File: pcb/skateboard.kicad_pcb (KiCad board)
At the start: 4 copper layers, 86.2 x 84.8 mm, 177 parts, among them J1 RC555, J10 PH_2.0, J11 adc_sensor2, J12 adc_sensor1, J13 Conn_01x01_Pin, J14 Conn_01x01_Pin, J15 Conn_01x01_Pin, J16 Conn_01x01_Pin, J2 pa1010d, J3 can_sensor, J4 USB_C_Receptacle_USB2.0_16P, J5 UART, J6 TB_MOTOR, J7 PH_2.0, J8 power, J9 TB_MOTOR, Q1 AO3401A, Q4 BTN8982TA, Q5 BTN8982TA, Q6 BTN8982TA, Q7 BTN8982TA, Q8 BTN8982TA, Q9 BTN8982TA, SW1 SW_SPST, SW2 BOOT, SW3 EN, U1 HX711, U10 INA240A2PW, U11 INA240A2PW, U2 SIT1042AQT/3, U3 ESP32-S3-WROOM-1, U4 LMR16030SDDAR, U5 LMR16030SDDAR, U6 LMR16030SDDAR, U7 INA240A2PW, U8 INA240A2PW, U9 HX711

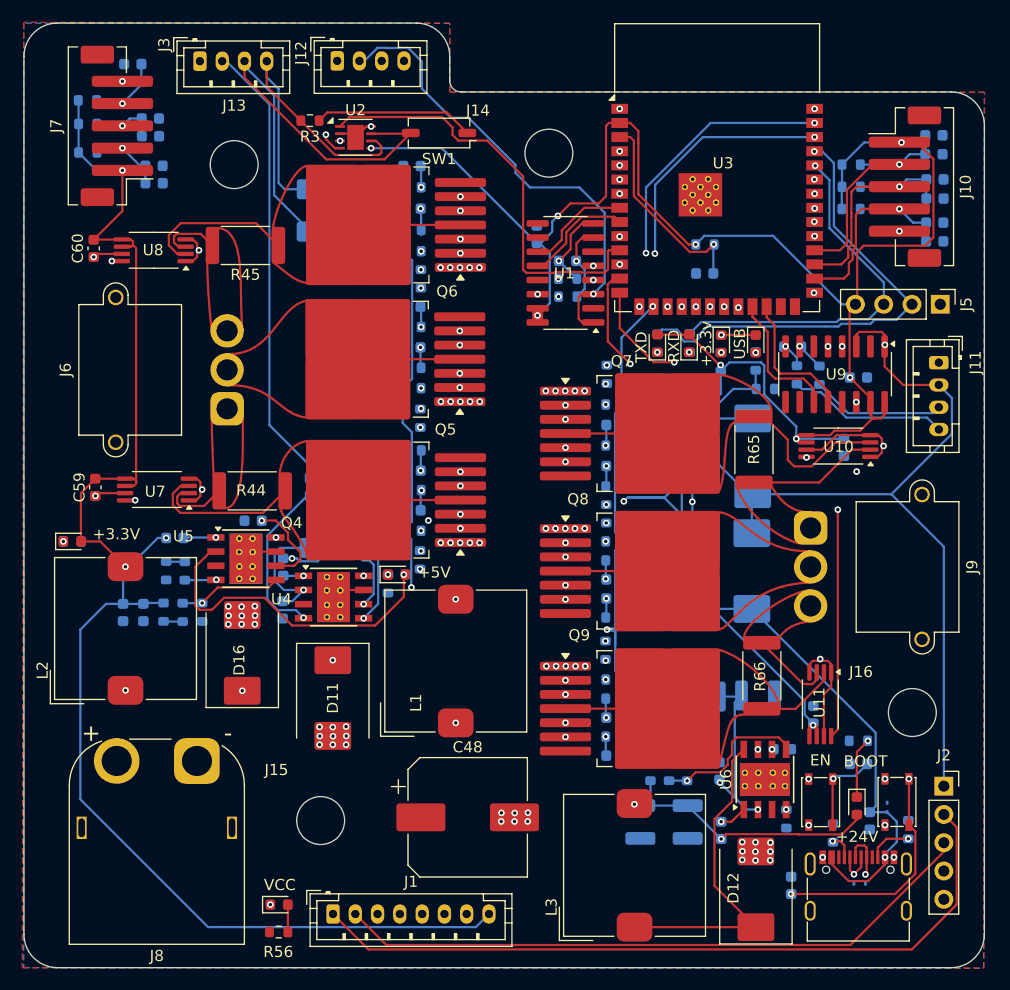
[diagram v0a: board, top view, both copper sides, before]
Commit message: update
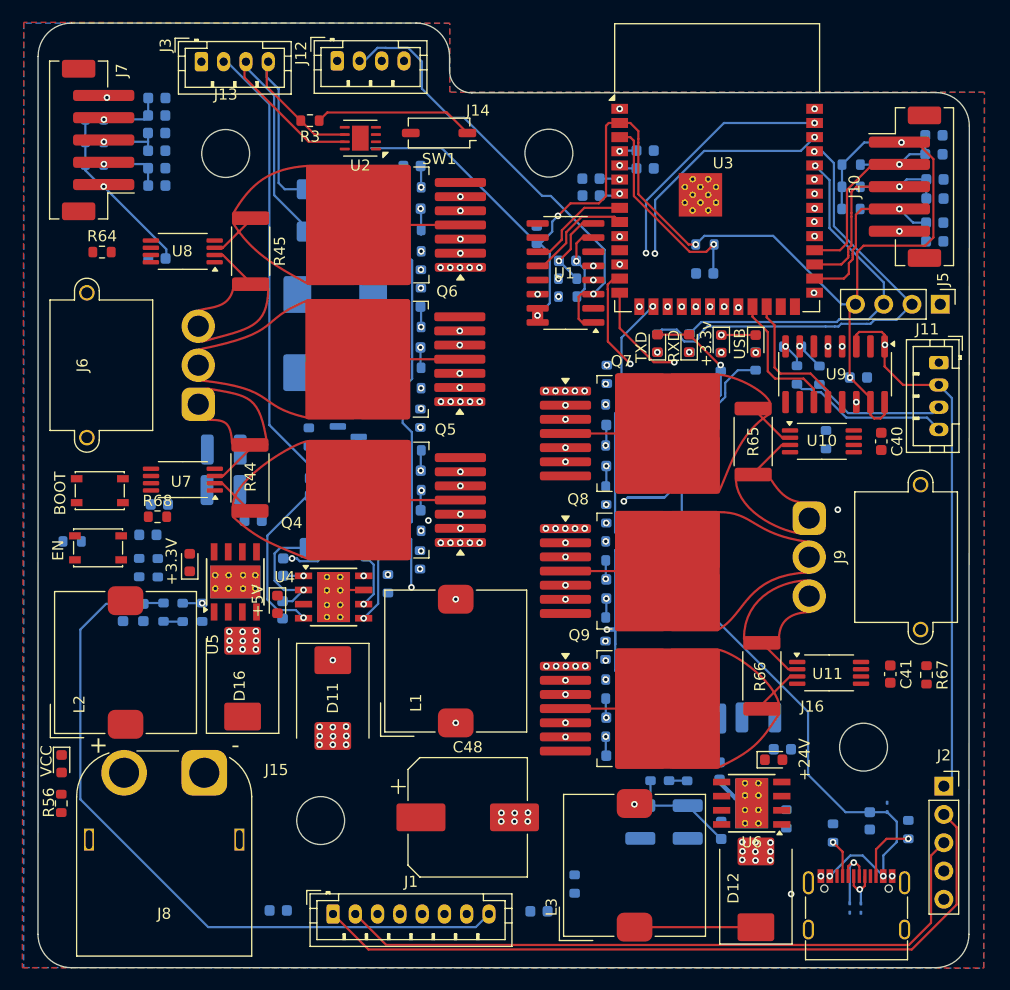
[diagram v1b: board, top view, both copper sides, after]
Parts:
- added C21: 100nf, Capacitor_SMD:C_0603_1608Metric, B.Cu at (137.9, 84.7)
- added C24: 100nf, Capacitor_SMD:C_0603_1608Metric, B.Cu at (142.8, 82.2)
- added C28: 100nf, Capacitor_SMD:C_0603_1608Metric, B.Cu at (137.9, 86.2)
- added C6: 100nf, Capacitor_SMD:C_0603_1608Metric, B.Cu at (142.8, 83.8)
- added R64: 200k, Resistor_SMD:R_0603_1608Metric, F.Cu at (94.0, 91.3)
- added R67: 200k, Resistor_SMD:R_0603_1608Metric, F.Cu at (168.1, 129.3)
- added R68: 200k, Resistor_SMD:R_0603_1608Metric, F.Cu at (99.0, 115.1)
- added R69: 200k, Resistor_SMD:R_0603_1608Metric, B.Cu at (159.0, 108.1)
- C12, C13, C19: value 100nF/16v -> 100nF
- C40, C41: moved to F.Cu
- C59, C60: moved to B.Cu
- C8: value 100nf/50v -> 100nf
- D4, D5: value MBR120VLSFT1G -> B560C
- moved SW2 76.8 mm to (93.8, 112.7), turned to 0 degrees
- moved SW3 68.8 mm to (93.7, 117.9), turned to 0 degrees
- moved C43 46.1 mm to (109.8, 150.4), turned to 0 degrees
- moved D4 41.4 mm to (115.0, 102.1), turned to 180 degrees
- moved C15 41.2 mm to (105.0, 109.0)
- moved C14 41.2 mm to (104.9, 112.7)
- moved R7 41.2 mm to (112.6, 107.9), turned to 90 degrees
- moved D5 40.2 mm to (115.0, 95.1), turned to 180 degrees
- moved C45 31.6 mm to (133.3, 150.5), turned to 0 degrees
- moved Q1 31.0 mm to (116.1, 107.9), turned to 0 degrees
- moved R19 28.5 mm to (136.5, 148.0), turned to -90 degrees
- moved 3.3V4 23.3 mm to (90.4, 137.2), turned to -90 degrees
- moved R56 22.7 mm to (90.4, 140.8), turned to 90 degrees
- moved D14 11.0 mm to (109.8, 122.9), turned to -90 degrees
- moved D17 10.7 mm to (101.9, 119.2), turned to 90 degrees
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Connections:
- Q4 pad 4: Net-(U7--) -> Net-(U7-+)
- Q4 pad 8: Net-(U7--) -> Net-(U7-+)
- Q6 pad 4: Net-(U8-+) -> Net-(U8--)
- Q6 pad 8: Net-(U8-+) -> Net-(U8--)
- Q7 pad 4: Net-(U10--) -> Net-(U10-+)
- Q7 pad 8: Net-(U10--) -> Net-(U10-+)
- Q9 pad 4: Net-(U11-+) -> Net-(U11--)
- Q9 pad 8: Net-(U11-+) -> Net-(U11--)
- R44 pad 2: Net-(U7--) -> Net-(U7-+)
- R45 pad 1: Net-(U8-+) -> Net-(U8--)
- R65 pad 2: Net-(U10--) -> Net-(U10-+)
- R66 pad 1: Net-(U11-+) -> Net-(U11--)
- U10 pad 2: Net-(J9-Pin_1) -> Net-(U10-+)
- U10 pad 3: Net-(U10--) -> Net-(J9-Pin_1)
- U10 pad 6: +3.3V -> Net-(U10-REF2)
- U11 pad 2: Net-(U11-+) -> Net-(J9-Pin_3)
- U11 pad 3: Net-(J9-Pin_3) -> Net-(U11--)
- U11 pad 6: +3.3V -> Net-(U11-REF2)
- U7 pad 2: Net-(J6-Pin_1) -> Net-(U7-+)
- U7 pad 3: Net-(U7--) -> Net-(J6-Pin_1)
- U7 pad 6: +3.3V -> Net-(U7-REF2)
- U8 pad 2: Net-(U8-+) -> Net-(J6-Pin_3)
- U8 pad 3: Net-(J6-Pin_3) -> Net-(U8--)
- U8 pad 6: +3.3V -> Net-(U8-REF2)
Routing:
- net +3.3V: track 379.5 -> 273.0 mm, vias 14 -> 9
- net +5V: track 217.4 -> 159.7 mm, vias 4 -> 2
- net EN: track 84.3 -> 37.4 mm, vias 2 -> 1
- net GND: track 51.5 -> 12.3 mm, vias 90 -> 76
- net TXD_SENSOR: track 38.4 -> 0.00 mm
- net Net-(D16-K): track 25.5 -> 0.00 mm, vias 3 -> 0
- net Net-(U10--): track 23.4 -> 0.00 mm
- net Net-(U8-+): track 23.0 -> 0.00 mm
- net Net-(U7--): track 20.8 -> 0.00 mm
- net /foc2/A1: track 57.2 -> 38.5 mm
- net Net-(D12-K): track 29.5 -> 10.9 mm
- net /mcu/Battery_5V: track 80.2 -> 62.4 mm, vias 3 -> 2
- net Net-(U11-+): track 14.2 -> 0.00 mm
- net Net-(U8--): track 0.00 -> 13.6 mm
- net Net-(U10-+): track 0.00 -> 13.5 mm
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- removed copper zone on F.Cu, net Net-(J6-Pin_1)
- removed copper zone on F.Cu, net Net-(J6-Pin_2)
- removed copper zone on F.Cu, net Net-(J6-Pin_3)
- removed copper zone on F.Cu, net Net-(J9-Pin_1)
- removed copper zone on F.Cu, net Net-(J9-Pin_2)
- removed copper zone on F.Cu, net Net-(J9-Pin_3)
- removed copper zone on F.Cu, net Net-(U10--)
- removed copper zone on F.Cu, net Net-(U11-+)
- removed copper zone on F.Cu, net Net-(U7--)
- removed copper zone on F.Cu, net Net-(U8-+)
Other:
- board size 86.2 x 84.8 mm -> 83.6 x 84.8 mm
